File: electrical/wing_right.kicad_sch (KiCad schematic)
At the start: 7 parts

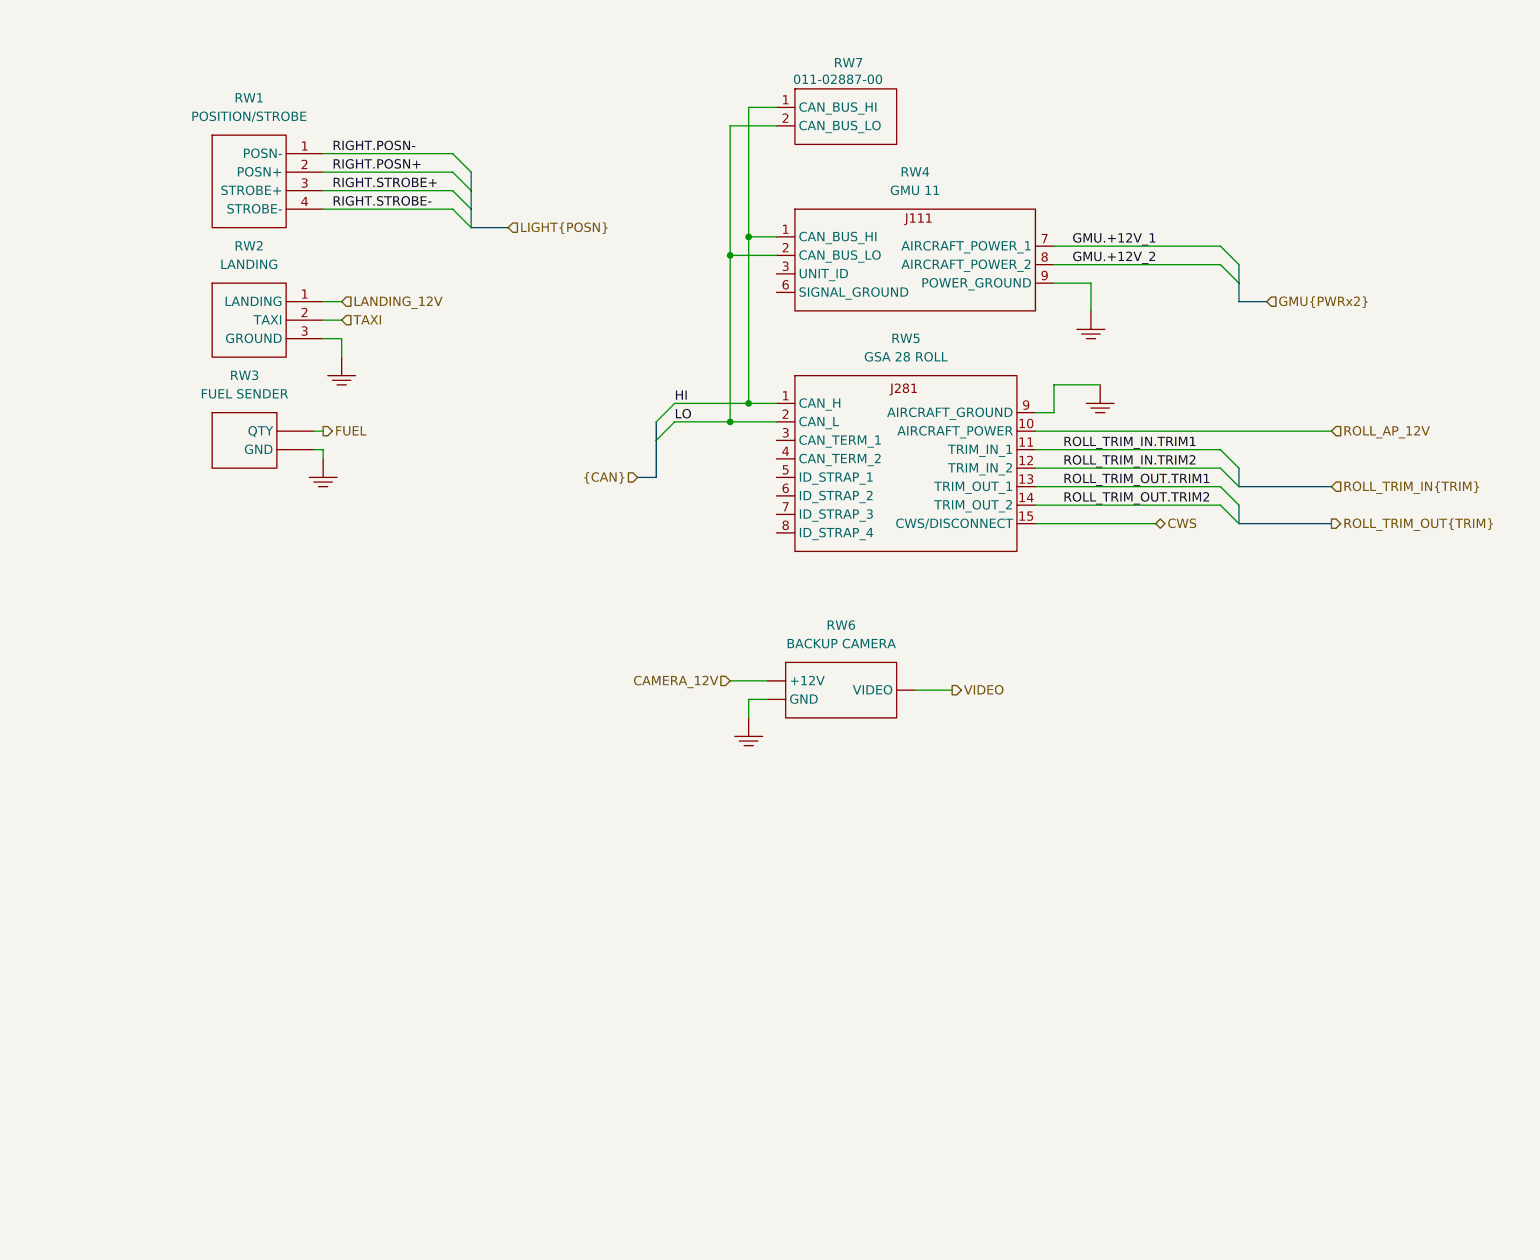
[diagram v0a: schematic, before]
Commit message: 🎮 Working on electrical schematic
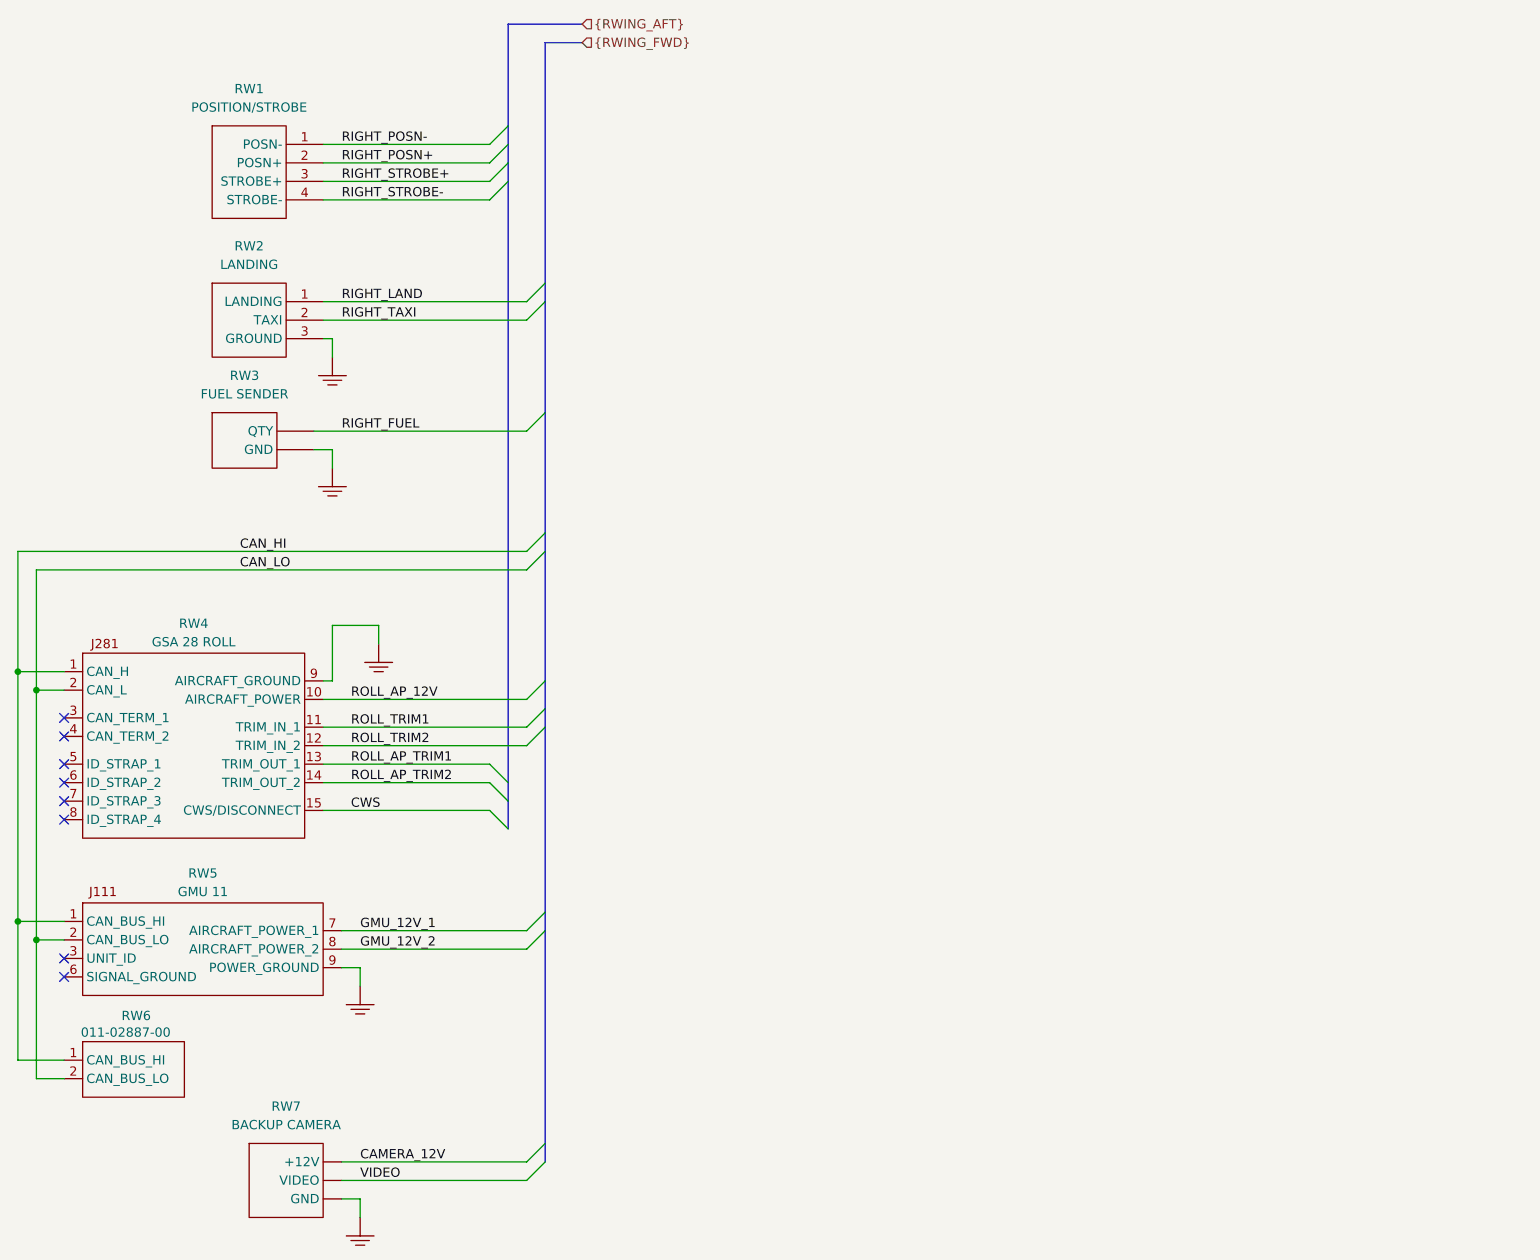
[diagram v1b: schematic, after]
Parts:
- renumbered RW5 to RW4, RW4 to RW5, RW7 to RW6, RW6 to RW7
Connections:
- net GND: now also RW3.2 (GND); no longer RW3. (GND)
- removed net FUEL: RW3. (GND)
- net GMU.+12V_1 renamed GMU_12V_1
- net GMU.+12V_2 renamed GMU_12V_2
- net HI renamed CAN_HI
- net LANDING_12V renamed RIGHT_LAND
- net LO renamed CAN_LO
- net RIGHT.POSN+ renamed RIGHT_POSN+
- net RIGHT.POSN- renamed RIGHT_POSN-
- net RIGHT.STROBE+ renamed RIGHT_STROBE+
- net RIGHT.STROBE- renamed RIGHT_STROBE-
- net ROLL_TRIM_IN.TRIM1 renamed ROLL_TRIM1
- net ROLL_TRIM_IN.TRIM2 renamed ROLL_TRIM2
- net ROLL_TRIM_OUT.TRIM1 renamed ROLL_AP_TRIM1
- net ROLL_TRIM_OUT.TRIM2 renamed ROLL_AP_TRIM2
- net TAXI renamed RIGHT_TAXI
- new net RIGHT_FUEL: RW3.1 (QTY)
- no-connect marks 0 -> 8
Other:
- moved on the sheet: RW4, RW5, RW6, RW7
